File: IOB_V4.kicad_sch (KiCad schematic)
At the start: 10 parts, among them J1 Conn_01x02, J18 Conn_01x10, J2 Conn_01x03, J20 Conn_01x10, U1 REF3033

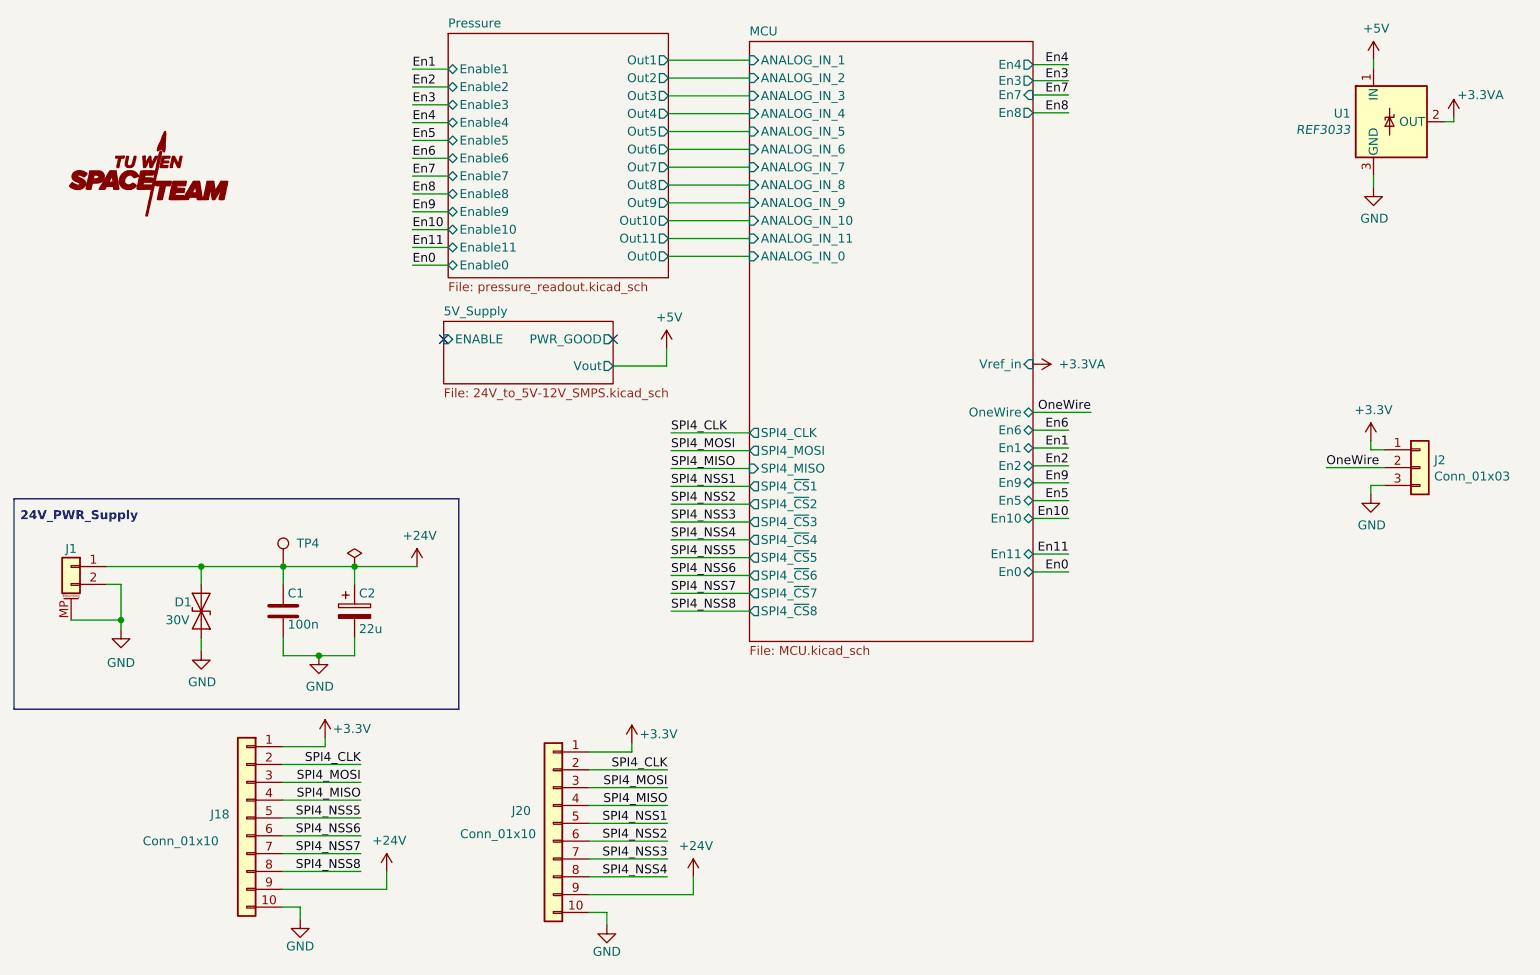
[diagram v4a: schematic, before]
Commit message: WIP
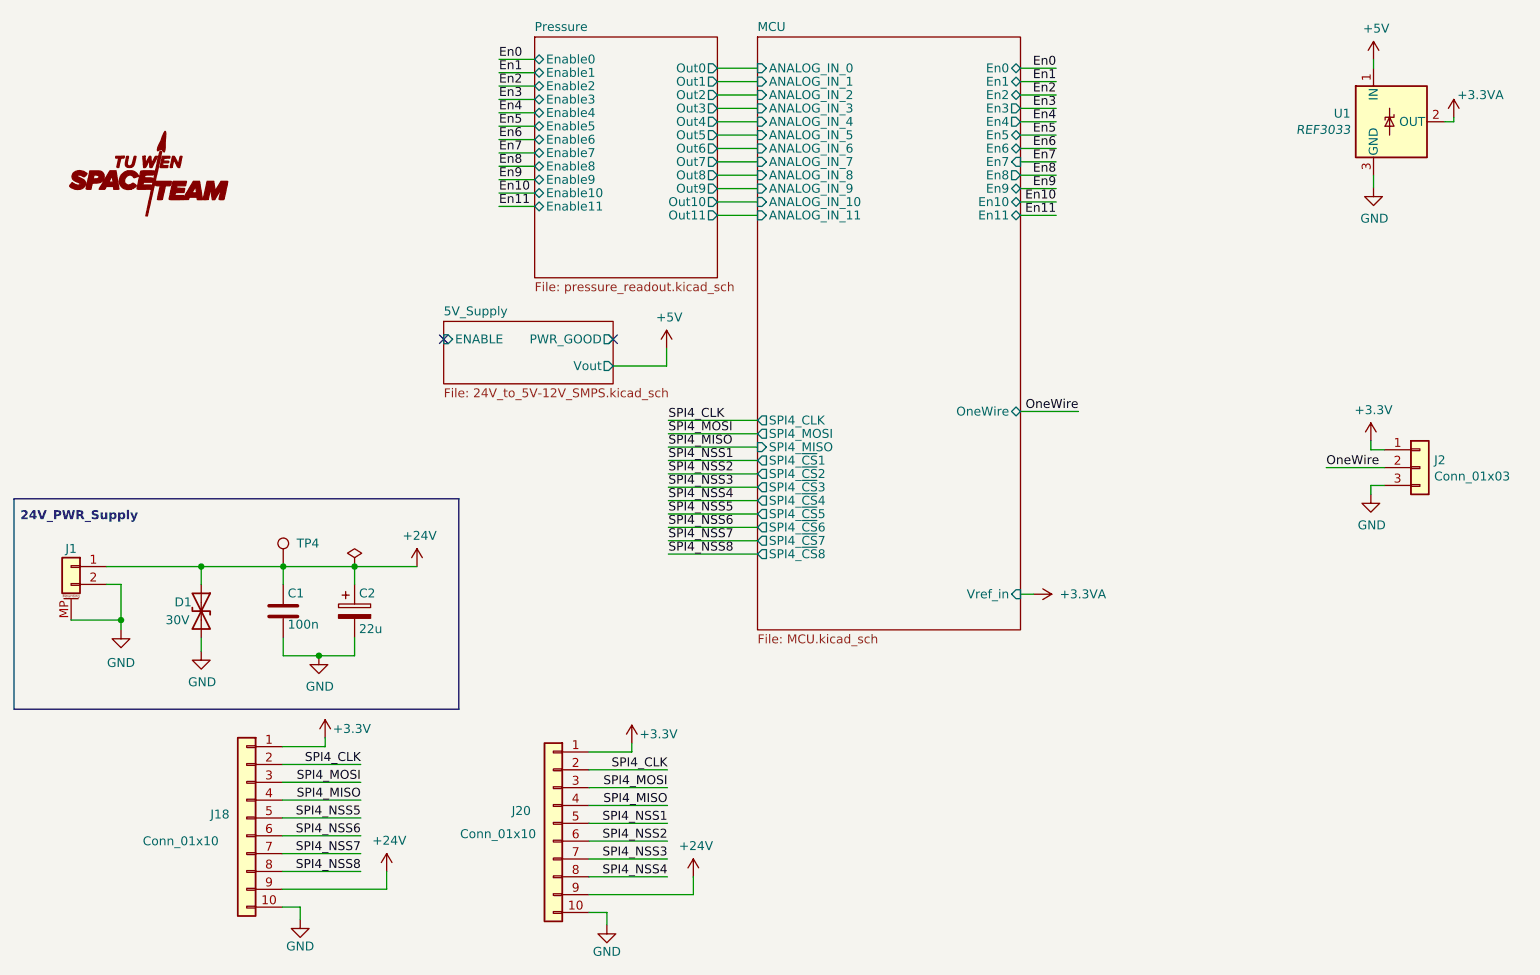
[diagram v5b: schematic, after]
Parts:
- C2: symbol Device:CP -> Device:C_Polarized
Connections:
- net +3V3 renamed +3.3V
